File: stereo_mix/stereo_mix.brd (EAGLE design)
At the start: 49 x 100 mm, 16 parts, among them U1 THONKICONNNEW, U2 THONKICONNNEW, U3 THONKICONNNEW, U4 THONKICONNNEW, U5 THONKICONNNEW, U6 THONKICONNNEW, U7 THONKICONNNEW, U8 THONKICONNNEW

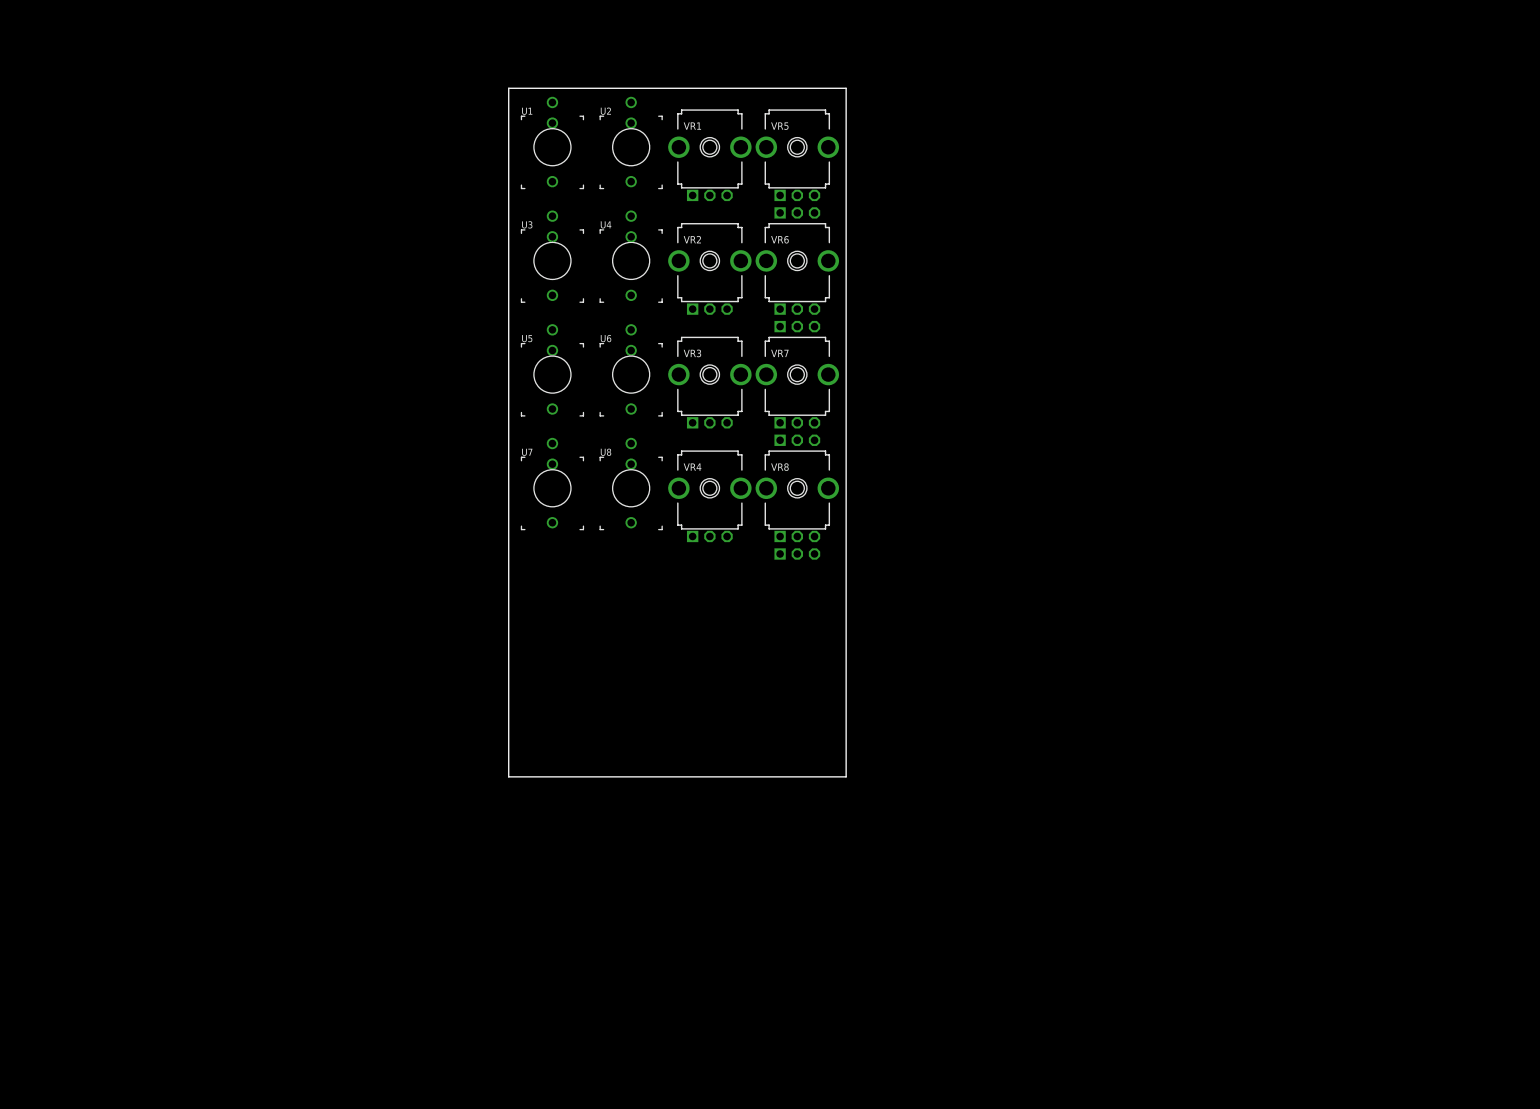
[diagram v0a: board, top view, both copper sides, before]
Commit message: Start implementation of stereo_mixer
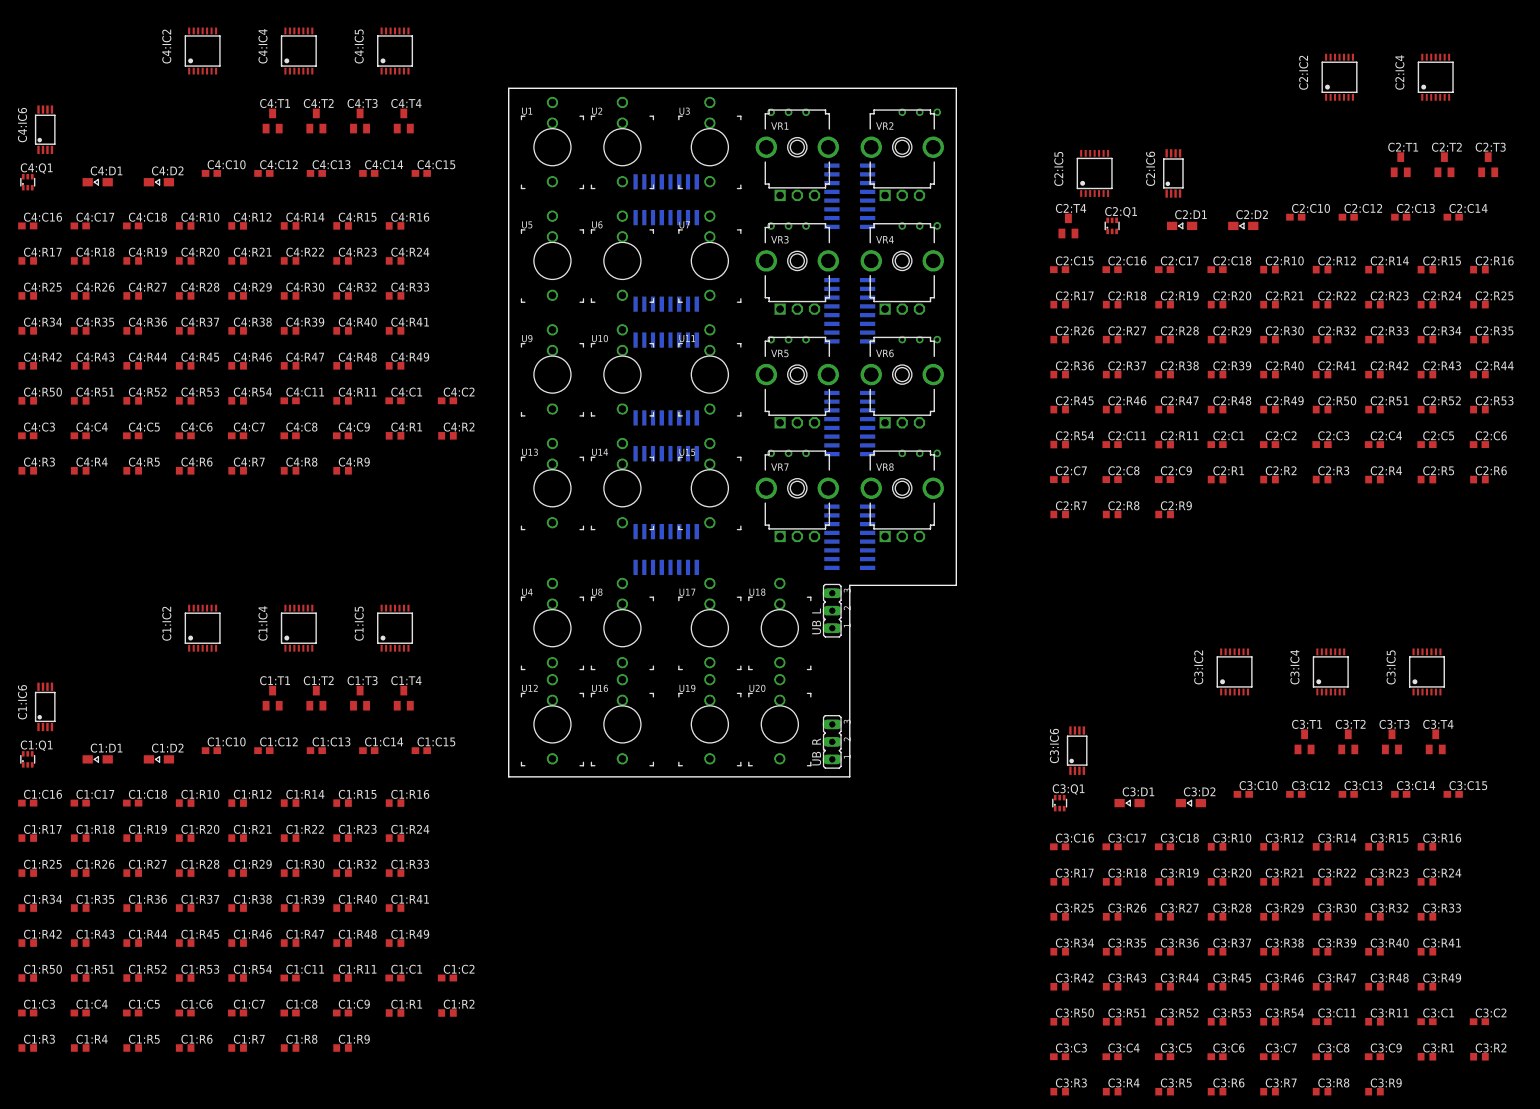
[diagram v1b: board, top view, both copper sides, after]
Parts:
- added C1:C1, C1:C3, C1:C5, C1:C6, C2:C1, C2:C3, C2:C5, C2:C6, C3:C1, C3:C3, C3:C5, C3:C6, C4:C1, C4:C3, C4:C5, C4:C6: 100pF, rcl:C0603
- added C1:C10, C1:C11, C1:C12, C1:C13, C1:C14, C1:C15, C1:C16, C1:C17, C1:C18, C1:C7, C1:C8, C1:C9, C2:C10, C2:C11, C2:C12, C2:C13, C2:C14, C2:C15, C2:C16, C2:C17, C2:C18, C2:C7, C2:C8, C2:C9, C3:C10, C3:C11, C3:C12, C3:C13, C3:C14, C3:C15, C3:C16, C3:C17, C3:C18, C3:C7, C3:C8, C3:C9, C4:C10, C4:C11, C4:C12, C4:C13, C4:C14, C4:C15, C4:C16, C4:C17, C4:C18, C4:C7, C4:C8, C4:C9: 100nF, rcl:C0603
- added C1:C2, C1:C4, C2:C2, C2:C4, C3:C2, C3:C4, C4:C2, C4:C4: 22pF, rcl:C0603
- added C1:D1, C1:D2, C2:D1, C2:D2, C3:D1, C3:D2, C4:D1, C4:D2: 1N4148, diode:SOD323-W
- added C1:IC1, C1:IC3, C2:IC1, C2:IC3, C3:IC1, C3:IC3, C4:IC1, C4:IC3: LM13700M, ota:SO16
- added C1:IC2, C1:IC4, C1:IC5, C2:IC2, C2:IC4, C2:IC5, C3:IC2, C3:IC4, C3:IC5, C4:IC2, C4:IC4, C4:IC5: TL084PW, op-amp:TSSOP14
- added C1:IC6, C2:IC6, C3:IC6, C4:IC6: TL082PW, op-amp:TSSOP8
- added C1:Q1, C2:Q1, C3:Q1, C4:Q1: BC847BS, transistor-small-signal:SOT363_PHILIPS
- added C1:R1, C1:R19, C2:R1, C2:R19, C3:R1, C3:R19, C4:R1, C4:R19: 22, rcl:R0603
- added C1:R10, C1:R15, C1:R28, C1:R33, C1:R43, C1:R44, C1:R45, C1:R46, C1:R49, C1:R50, C1:R51, C1:R52, C1:R53, C1:R54, C2:R10, C2:R15, C2:R28, C2:R33, C2:R43, C2:R44, C2:R45, C2:R46, C2:R49, C2:R50, C2:R51, C2:R52, C2:R53, C2:R54, C3:R10, C3:R15, C3:R28, C3:R33, C3:R43, C3:R44, C3:R45, C3:R46, C3:R49, C3:R50, C3:R51, C3:R52, C3:R53, C3:R54, C4:R10, C4:R15, C4:R28, C4:R33, C4:R43, C4:R44, C4:R45, C4:R46, C4:R49, C4:R50, C4:R51, C4:R52, C4:R53, C4:R54: 100k, rcl:R0603
- added C1:R11, C1:R29, C2:R11, C2:R29, C3:R11, C3:R29, C4:R11, C4:R29: 680, rcl:R0603
- added C1:R12, C1:R30, C1:R37, C1:R39, C2:R12, C2:R30, C2:R37, C2:R39, C3:R12, C3:R30, C3:R37, C3:R39, C4:R12, C4:R30, C4:R37, C4:R39: 1M, rcl:R0603
- added C1:R13, C1:R31, C2:R13, C2:R31, C3:R13, C3:R31, C4:R13, C4:R31: 100k, rcl:RTRIMT93YA
- added C1:R14, C1:R32, C2:R14, C2:R32, C3:R14, C3:R32, C4:R14, C4:R32: 47k, rcl:R0603
- added C1:R16, C1:R34, C2:R16, C2:R34, C3:R16, C3:R34, C4:R16, C4:R34: 68k, rcl:R0603
- added C1:R17, C1:R27, C1:R35, C1:R9, C2:R17, C2:R27, C2:R35, C2:R9, C3:R17, C3:R27, C3:R35, C3:R9, C4:R17, C4:R27, C4:R35, C4:R9: 15k, rcl:R0603
- added C1:R18, C1:R36, C2:R18, C2:R36, C3:R18, C3:R36, C4:R18, C4:R36: 680k, rcl:R0603
- added C1:R2, C1:R20, C2:R2, C2:R20, C3:R2, C3:R20, C4:R2, C4:R20: 470, rcl:R0603
- added C1:R21, C1:R3, C2:R21, C2:R3, C3:R21, C3:R3, C4:R21, C4:R3: 510, rcl:R0603
- added C1:R22, C1:R4, C2:R22, C2:R4, C3:R22, C3:R4, C4:R22, C4:R4: 21k, rcl:R0603
- added C1:R23, C1:R5, C2:R23, C2:R5, C3:R23, C3:R5, C4:R23, C4:R5: 12k, rcl:R0603
- added C1:R24, C1:R6, C2:R24, C2:R6, C3:R24, C3:R6, C4:R24, C4:R6: 7k2, rcl:R0603
- added C1:R25, C1:R7, C2:R25, C2:R7, C3:R25, C3:R7, C4:R25, C4:R7: 6k8, rcl:R0603
- added C1:R26, C1:R8, C2:R26, C2:R8, C3:R26, C3:R8, C4:R26, C4:R8: 560, rcl:R0603
- added C1:R38, C2:R38, C3:R38, C4:R38: 1k, rcl:R0603
- added C1:R40, C2:R40, C3:R40, C4:R40: 10k, rcl:R0603
- added C1:R41, C2:R41, C3:R41, C4:R41: 10M, rcl:R0603
- added C1:R42, C2:R42, C3:R42, C4:R42: 1k5, rcl:R0603
- added C1:R47, C1:R48, C2:R47, C2:R48, C3:R47, C3:R48, C4:R47, C4:R48: 200k, rcl:R0603
- added C1:T1, C1:T2, C1:T3, C1:T4, C2:T1, C2:T2, C2:T3, C2:T4, C3:T1, C3:T2, C3:T3, C3:T4, C4:T1, C4:T2, C4:T3, C4:T4: 3906, transistor-neu-to92:SOT23-BEC
- added U10, U11, U12, U13, U14, U15, U16, U17, U18, U19, U20, U9: THONKICONNNEW, MusicThingModular:WQP-PJ301M-12_JACK
- added UB_L, UB_R: (no value), jumper:JP2
- VR5, VR6, VR7, VR8: device MusicThingModular:DUAL_9MM_SNAP-IN_POT -> MusicThingModular:9MM_SNAP-IN_POT
- moved U4 54.6 mm to (6.35, 21.6)
- moved VR4 43.3 mm to (57.1, 74.9)
- moved U7 40.2 mm to (29.2, 74.9)
- moved VR5 33.0 mm to (41.9, 58.4)
- moved VR2 32.5 mm to (57.1, 91.4)
- moved U3 28.2 mm to (29.2, 91.4)
- moved VR6 22.5 mm to (57.1, 58.4)
- moved VR3 20.8 mm to (41.9, 74.9)
- moved U8 20.4 mm to (16.5, 21.6)
- moved U6 16.6 mm to (16.5, 74.9)
- moved U5 16.5 mm to (6.35, 74.9)
- moved VR7 16.5 mm to (41.9, 41.9)
- moved VR8 15.2 mm to (57.1, 41.9)
- moved VR1 12.7 mm to (41.9, 91.4)
- moved U2 1.27 mm to (16.5, 91.4)
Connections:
- new net +12V: C1:C10.2, C1:C11.2, C1:C12.2, C1:C7.2, C1:C8.2, C1:C9.2, C1:IC1.11, C1:IC2.4, C1:IC3.11, C1:IC4.4, C1:IC5.4, C1:IC6.8, C1:R13.1, C1:R23.1, C1:R31.1, C1:R37.2, C1:R41.2, C1:R5.1, C2:C10.2, C2:C11.2, C2:C12.2, C2:C7.2, C2:C8.2, C2:C9.2, C2:IC1.11, C2:IC2.4, C2:IC3.11, C2:IC4.4, C2:IC5.4, C2:IC6.8, C2:R13.1, C2:R23.1, C2:R31.1, C2:R37.2, C2:R41.2, C2:R5.1, C3:C10.2, C3:C11.2, C3:C12.2, C3:C7.2, C3:C8.2, C3:C9.2, C3:IC1.11, C3:IC2.4, C3:IC3.11, C3:IC4.4, C3:IC5.4, C3:IC6.8, C3:R13.1, C3:R23.1, C3:R31.1, C3:R37.2, C3:R41.2, C3:R5.1, C4:C10.2, C4:C11.2, C4:C12.2, C4:C7.2, C4:C8.2, C4:C9.2, C4:IC1.11, C4:IC2.4, C4:IC3.11, C4:IC4.4, C4:IC5.4, C4:IC6.8, C4:R13.1, C4:R23.1, C4:R31.1, C4:R37.2, C4:R41.2, C4:R5.1
- new net -12V: C1:C13.1, C1:C14.1, C1:C15.1, C1:C16.1, C1:C17.1, C1:C18.1, C1:IC1.6, C1:IC2.11, C1:IC3.6, C1:IC4.11, C1:IC5.11, C1:IC6.4, C1:R13.3, C1:R18.2, C1:R31.3, C1:R36.2, C2:C13.1, C2:C14.1, C2:C15.1, C2:C16.1, C2:C17.1, C2:C18.1, C2:IC1.6, C2:IC2.11, C2:IC3.6, C2:IC4.11, C2:IC5.11, C2:IC6.4, C2:R13.3, C2:R18.2, C2:R31.3, C2:R36.2, C3:C13.1, C3:C14.1, C3:C15.1, C3:C16.1, C3:C17.1, C3:C18.1, C3:IC1.6, C3:IC2.11, C3:IC3.6, C3:IC4.11, C3:IC5.11, C3:IC6.4, C3:R13.3, C3:R18.2, C3:R31.3, C3:R36.2, C4:C13.1, C4:C14.1, C4:C15.1, C4:C16.1, C4:C17.1, C4:C18.1, C4:IC1.6, C4:IC2.11, C4:IC3.6, C4:IC4.11, C4:IC5.11, C4:IC6.4, C4:R13.3, C4:R18.2, C4:R31.3, C4:R36.2
- new net C1:N$1: C1:IC1.4, C1:R1.2
- new net C1:N$10: C1:R8.1, C1:R9.2
- new net C1:N$11: C1:IC2.7, C1:R10.1, C1:R8.2
- new net C1:N$12: C1:C1.1, C1:IC1.13, C1:R12.2, C1:R14.1
- new net C1:N$13: C1:IC1.14, C1:R10.2, C1:R11.2
- new net C1:N$14: C1:R12.1, C1:R13.2
- new net C1:N$15: C1:C2.1, C1:IC2.9, C1:R15.1, C1:R16.2
- new net C1:N$16: C1:C1.2, C1:IC1.12, C1:IC2.10, C1:R14.2
- new net C1:N$17: C1:IC1.16, C1:R17.2
- new net C1:N$18: C1:R17.1, C1:R18.1, C1:T2.C
- new net C1:N$19: C1:IC2.13, C1:IC2.14, C1:T2.B
- new net C1:N$2: C1:R1.1, C1:R2.2
- new net C1:N$20: C1:IC3.4, C1:R19.2
- new net C1:N$21: C1:R19.1, C1:R20.2
- new net C1:N$22: C1:IC3.3, C1:R21.2, C1:R22.2
- new net C1:N$23: C1:IC3.2, C1:R23.2
- new net C1:N$24: C1:IC3.1, C1:R24.2
- new net C1:N$25: C1:R24.1, C1:T3.C
- new net C1:N$26: C1:D2.A, C1:IC4.1, C1:T3.B
- new net C1:N$27: C1:D2.C, C1:IC4.2, C1:R25.2, C1:T3.E
- new net C1:N$28: C1:IC3.5, C1:IC4.6, C1:R27.1
- new net C1:N$29: C1:R26.1, C1:R27.2
- new net C1:N$3: C1:IC1.3, C1:R3.2, C1:R4.2
- new net C1:N$30: C1:IC4.7, C1:R26.2, C1:R28.1
- new net C1:N$31: C1:IC3.14, C1:R28.2, C1:R29.2
- new net C1:N$32: C1:C3.1, C1:IC3.13, C1:R30.2, C1:R32.1
- new net C1:N$33: C1:R30.1, C1:R31.2
- new net C1:N$34: C1:C3.2, C1:IC3.12, C1:IC4.10, C1:R32.2
- new net C1:N$35: C1:C4.1, C1:IC4.9, C1:R33.1, C1:R34.2
- new net C1:N$36: C1:IC3.16, C1:R35.2
- new net C1:N$37: C1:R35.1, C1:R36.1, C1:T4.C
- new net C1:N$38: C1:IC4.13, C1:IC4.14, C1:T4.B
- new net C1:N$39: C1:IC5.1, C1:IC5.2, C1:R39.2
- new net C1:N$4: C1:IC1.1, C1:R6.2
- new net C1:N$40: C1:IC5.3, C1:R37.1, C1:R38.1
- new net C1:N$41: C1:C5.1, C1:IC5.6, C1:R39.1, C1:R40.1
- new net C1:N$42: C1:C5.2, C1:IC5.7, C1:Q1.2, C1:R40.2
- new net C1:N$43: C1:IC6.5, C1:R43.2, C1:R44.2
- new net C1:N$44: C1:C6.1, C1:IC5.9, C1:Q1.6, C1:R41.1
- new net C1:N$45: C1:IC6.6, C1:R45.2, C1:R46.1
- new net C1:N$46: C1:Q1.1, C1:Q1.4, C1:R42.2
- new net C1:N$47: C1:IC6.2, C1:R47.1, C1:R48.2
- new net C1:N$48: C1:IC5.13, C1:R51.2, C1:R52.1
- new net C1:N$5: C1:IC1.2, C1:R5.2
- new net C1:N$50: C1:IC6.3, C1:R49.2, C1:R50.2
- new net C1:N$6: C1:R6.1, C1:T1.C
- new net C1:N$7: C1:D1.A, C1:IC2.1, C1:T1.B
- new net C1:N$8: C1:D1.C, C1:IC2.2, C1:R7.2, C1:T1.E
- new net C1:N$9: C1:IC1.5, C1:IC2.6, C1:R9.1
- new net C1:OUT_L: C1:C2.2, C1:IC2.8, C1:R15.2
- new net C1:OUT_R: C1:C4.2, C1:IC4.8, C1:R33.2
- new net C1:PAN_CV: C1:IC5.14, C1:R45.1, C1:R49.1, C1:R51.1
- new net C1:PAN_CV_L: C1:IC6.7, C1:R46.2, C1:R7.1
- new net C1:PAN_CV_R: C1:IC6.1, C1:R25.1, C1:R47.2
- new net C1:REF_5: C1:R43.1, C1:R50.1
- new net C1:VOLUME_CV_LOG: C1:C6.2, C1:IC2.12, C1:IC4.12, C1:IC5.8, C1:R42.1
- new net C2:N$1: C2:IC1.4, C2:R1.2
- new net C2:N$10: C2:R8.1, C2:R9.2
- new net C2:N$11: C2:IC2.7, C2:R10.1, C2:R8.2
- new net C2:N$12: C2:C1.1, C2:IC1.13, C2:R12.2, C2:R14.1
- new net C2:N$13: C2:IC1.14, C2:R10.2, C2:R11.2
- new net C2:N$14: C2:R12.1, C2:R13.2
- new net C2:N$15: C2:C2.1, C2:IC2.9, C2:R15.1, C2:R16.2
- new net C2:N$16: C2:C1.2, C2:IC1.12, C2:IC2.10, C2:R14.2
- new net C2:N$17: C2:IC1.16, C2:R17.2
- new net C2:N$18: C2:R17.1, C2:R18.1, C2:T2.C
- new net C2:N$19: C2:IC2.13, C2:IC2.14, C2:T2.B
- new net C2:N$2: C2:R1.1, C2:R2.2
- new net C2:N$20: C2:IC3.4, C2:R19.2
- new net C2:N$21: C2:R19.1, C2:R20.2
- new net C2:N$22: C2:IC3.3, C2:R21.2, C2:R22.2
- new net C2:N$23: C2:IC3.2, C2:R23.2
- new net C2:N$24: C2:IC3.1, C2:R24.2
- new net C2:N$25: C2:R24.1, C2:T3.C
- new net C2:N$26: C2:D2.A, C2:IC4.1, C2:T3.B
- new net C2:N$27: C2:D2.C, C2:IC4.2, C2:R25.2, C2:T3.E
- new net C2:N$28: C2:IC3.5, C2:IC4.6, C2:R27.1
- new net C2:N$29: C2:R26.1, C2:R27.2
- new net C2:N$3: C2:IC1.3, C2:R3.2, C2:R4.2
- new net C2:N$30: C2:IC4.7, C2:R26.2, C2:R28.1
- new net C2:N$31: C2:IC3.14, C2:R28.2, C2:R29.2
- new net C2:N$32: C2:C3.1, C2:IC3.13, C2:R30.2, C2:R32.1
- new net C2:N$33: C2:R30.1, C2:R31.2
- new net C2:N$34: C2:C3.2, C2:IC3.12, C2:IC4.10, C2:R32.2
- new net C2:N$35: C2:C4.1, C2:IC4.9, C2:R33.1, C2:R34.2
- new net C2:N$36: C2:IC3.16, C2:R35.2
- new net C2:N$37: C2:R35.1, C2:R36.1, C2:T4.C
- new net C2:N$38: C2:IC4.13, C2:IC4.14, C2:T4.B
- new net C2:N$39: C2:IC5.1, C2:IC5.2, C2:R39.2
- new net C2:N$4: C2:IC1.1, C2:R6.2
- new net C2:N$40: C2:IC5.3, C2:R37.1, C2:R38.1
- new net C2:N$41: C2:C5.1, C2:IC5.6, C2:R39.1, C2:R40.1
- new net C2:N$42: C2:C5.2, C2:IC5.7, C2:Q1.2, C2:R40.2
- new net C2:N$43: C2:IC6.5, C2:R43.2, C2:R44.2
- new net C2:N$44: C2:C6.1, C2:IC5.9, C2:Q1.6, C2:R41.1
- new net C2:N$45: C2:IC6.6, C2:R45.2, C2:R46.1
- new net C2:N$46: C2:Q1.1, C2:Q1.4, C2:R42.2
- new net C2:N$47: C2:IC6.2, C2:R47.1, C2:R48.2
- new net C2:N$48: C2:IC5.13, C2:R51.2, C2:R52.1
- new net C2:N$5: C2:IC1.2, C2:R5.2
- new net C2:N$50: C2:IC6.3, C2:R49.2, C2:R50.2
- new net C2:N$6: C2:R6.1, C2:T1.C
- new net C2:N$7: C2:D1.A, C2:IC2.1, C2:T1.B
- new net C2:N$8: C2:D1.C, C2:IC2.2, C2:R7.2, C2:T1.E
- new net C2:N$9: C2:IC1.5, C2:IC2.6, C2:R9.1
- new net C2:OUT_L: C2:C2.2, C2:IC2.8, C2:R15.2
- new net C2:OUT_R: C2:C4.2, C2:IC4.8, C2:R33.2
- new net C2:PAN_CV: C2:IC5.14, C2:R45.1, C2:R49.1, C2:R51.1
- new net C2:PAN_CV_L: C2:IC6.7, C2:R46.2, C2:R7.1
- new net C2:PAN_CV_R: C2:IC6.1, C2:R25.1, C2:R47.2
- new net C2:REF_5: C2:R43.1, C2:R50.1
- new net C2:VOLUME_CV_LOG: C2:C6.2, C2:IC2.12, C2:IC4.12, C2:IC5.8, C2:R42.1
- new net C3:N$1: C3:IC1.4, C3:R1.2
- new net C3:N$10: C3:R8.1, C3:R9.2
- new net C3:N$11: C3:IC2.7, C3:R10.1, C3:R8.2
- new net C3:N$12: C3:C1.1, C3:IC1.13, C3:R12.2, C3:R14.1
- new net C3:N$13: C3:IC1.14, C3:R10.2, C3:R11.2
- new net C3:N$14: C3:R12.1, C3:R13.2
- new net C3:N$15: C3:C2.1, C3:IC2.9, C3:R15.1, C3:R16.2
- new net C3:N$16: C3:C1.2, C3:IC1.12, C3:IC2.10, C3:R14.2
- new net C3:N$17: C3:IC1.16, C3:R17.2
- new net C3:N$18: C3:R17.1, C3:R18.1, C3:T2.C
- new net C3:N$19: C3:IC2.13, C3:IC2.14, C3:T2.B
- new net C3:N$2: C3:R1.1, C3:R2.2
- new net C3:N$20: C3:IC3.4, C3:R19.2
- new net C3:N$21: C3:R19.1, C3:R20.2
- new net C3:N$22: C3:IC3.3, C3:R21.2, C3:R22.2
- new net C3:N$23: C3:IC3.2, C3:R23.2
- new net C3:N$24: C3:IC3.1, C3:R24.2
- new net C3:N$25: C3:R24.1, C3:T3.C
- new net C3:N$26: C3:D2.A, C3:IC4.1, C3:T3.B
- new net C3:N$27: C3:D2.C, C3:IC4.2, C3:R25.2, C3:T3.E
- new net C3:N$28: C3:IC3.5, C3:IC4.6, C3:R27.1
- new net C3:N$29: C3:R26.1, C3:R27.2
- new net C3:N$3: C3:IC1.3, C3:R3.2, C3:R4.2
- new net C3:N$30: C3:IC4.7, C3:R26.2, C3:R28.1
- new net C3:N$31: C3:IC3.14, C3:R28.2, C3:R29.2
- new net C3:N$32: C3:C3.1, C3:IC3.13, C3:R30.2, C3:R32.1
- new net C3:N$33: C3:R30.1, C3:R31.2
- new net C3:N$34: C3:C3.2, C3:IC3.12, C3:IC4.10, C3:R32.2
- new net C3:N$35: C3:C4.1, C3:IC4.9, C3:R33.1, C3:R34.2
- new net C3:N$36: C3:IC3.16, C3:R35.2
- new net C3:N$37: C3:R35.1, C3:R36.1, C3:T4.C
- new net C3:N$38: C3:IC4.13, C3:IC4.14, C3:T4.B
- new net C3:N$39: C3:IC5.1, C3:IC5.2, C3:R39.2
- new net C3:N$4: C3:IC1.1, C3:R6.2
- new net C3:N$40: C3:IC5.3, C3:R37.1, C3:R38.1
- new net C3:N$41: C3:C5.1, C3:IC5.6, C3:R39.1, C3:R40.1
- new net C3:N$42: C3:C5.2, C3:IC5.7, C3:Q1.2, C3:R40.2
- new net C3:N$43: C3:IC6.5, C3:R43.2, C3:R44.2
- new net C3:N$44: C3:C6.1, C3:IC5.9, C3:Q1.6, C3:R41.1
- new net C3:N$45: C3:IC6.6, C3:R45.2, C3:R46.1
- new net C3:N$46: C3:Q1.1, C3:Q1.4, C3:R42.2
- new net C3:N$47: C3:IC6.2, C3:R47.1, C3:R48.2
- new net C3:N$48: C3:IC5.13, C3:R51.2, C3:R52.1
- new net C3:N$5: C3:IC1.2, C3:R5.2
- new net C3:N$50: C3:IC6.3, C3:R49.2, C3:R50.2
- new net C3:N$6: C3:R6.1, C3:T1.C
- new net C3:N$7: C3:D1.A, C3:IC2.1, C3:T1.B
- new net C3:N$8: C3:D1.C, C3:IC2.2, C3:R7.2, C3:T1.E
- new net C3:N$9: C3:IC1.5, C3:IC2.6, C3:R9.1
- new net C3:OUT_L: C3:C2.2, C3:IC2.8, C3:R15.2
- new net C3:OUT_R: C3:C4.2, C3:IC4.8, C3:R33.2
- new net C3:PAN_CV: C3:IC5.14, C3:R45.1, C3:R49.1, C3:R51.1
- new net C3:PAN_CV_L: C3:IC6.7, C3:R46.2, C3:R7.1
- new net C3:PAN_CV_R: C3:IC6.1, C3:R25.1, C3:R47.2
- new net C3:REF_5: C3:R43.1, C3:R50.1
- new net C3:VOLUME_CV_LOG: C3:C6.2, C3:IC2.12, C3:IC4.12, C3:IC5.8, C3:R42.1
- new net C4:N$1: C4:IC1.4, C4:R1.2
- new net C4:N$10: C4:R8.1, C4:R9.2
- new net C4:N$11: C4:IC2.7, C4:R10.1, C4:R8.2
- new net C4:N$12: C4:C1.1, C4:IC1.13, C4:R12.2, C4:R14.1
- new net C4:N$13: C4:IC1.14, C4:R10.2, C4:R11.2
- new net C4:N$14: C4:R12.1, C4:R13.2
- new net C4:N$15: C4:C2.1, C4:IC2.9, C4:R15.1, C4:R16.2
- new net C4:N$16: C4:C1.2, C4:IC1.12, C4:IC2.10, C4:R14.2
- new net C4:N$17: C4:IC1.16, C4:R17.2
- new net C4:N$18: C4:R17.1, C4:R18.1, C4:T2.C
- new net C4:N$19: C4:IC2.13, C4:IC2.14, C4:T2.B
- new net C4:N$2: C4:R1.1, C4:R2.2
- new net C4:N$20: C4:IC3.4, C4:R19.2
- new net C4:N$21: C4:R19.1, C4:R20.2
- new net C4:N$22: C4:IC3.3, C4:R21.2, C4:R22.2
- new net C4:N$23: C4:IC3.2, C4:R23.2
- new net C4:N$24: C4:IC3.1, C4:R24.2
- new net C4:N$25: C4:R24.1, C4:T3.C
- new net C4:N$26: C4:D2.A, C4:IC4.1, C4:T3.B
- new net C4:N$27: C4:D2.C, C4:IC4.2, C4:R25.2, C4:T3.E
- new net C4:N$28: C4:IC3.5, C4:IC4.6, C4:R27.1
- new net C4:N$29: C4:R26.1, C4:R27.2
- new net C4:N$3: C4:IC1.3, C4:R3.2, C4:R4.2
- new net C4:N$30: C4:IC4.7, C4:R26.2, C4:R28.1
- new net C4:N$31: C4:IC3.14, C4:R28.2, C4:R29.2
- new net C4:N$32: C4:C3.1, C4:IC3.13, C4:R30.2, C4:R32.1
- new net C4:N$33: C4:R30.1, C4:R31.2
- new net C4:N$34: C4:C3.2, C4:IC3.12, C4:IC4.10, C4:R32.2
- new net C4:N$35: C4:C4.1, C4:IC4.9, C4:R33.1, C4:R34.2
- new net C4:N$36: C4:IC3.16, C4:R35.2
- new net C4:N$37: C4:R35.1, C4:R36.1, C4:T4.C
- new net C4:N$38: C4:IC4.13, C4:IC4.14, C4:T4.B
- new net C4:N$39: C4:IC5.1, C4:IC5.2, C4:R39.2
- new net C4:N$4: C4:IC1.1, C4:R6.2
- new net C4:N$40: C4:IC5.3, C4:R37.1, C4:R38.1
- new net C4:N$41: C4:C5.1, C4:IC5.6, C4:R39.1, C4:R40.1
- new net C4:N$42: C4:C5.2, C4:IC5.7, C4:Q1.2, C4:R40.2
- new net C4:N$43: C4:IC6.5, C4:R43.2, C4:R44.2
- new net C4:N$44: C4:C6.1, C4:IC5.9, C4:Q1.6, C4:R41.1
- new net C4:N$45: C4:IC6.6, C4:R45.2, C4:R46.1
- new net C4:N$46: C4:Q1.1, C4:Q1.4, C4:R42.2
- new net C4:N$47: C4:IC6.2, C4:R47.1, C4:R48.2
- new net C4:N$48: C4:IC5.13, C4:R51.2, C4:R52.1
- new net C4:N$5: C4:IC1.2, C4:R5.2
- new net C4:N$50: C4:IC6.3, C4:R49.2, C4:R50.2
- new net C4:N$6: C4:R6.1, C4:T1.C
- new net C4:N$7: C4:D1.A, C4:IC2.1, C4:T1.B
- new net C4:N$8: C4:D1.C, C4:IC2.2, C4:R7.2, C4:T1.E
- new net C4:N$9: C4:IC1.5, C4:IC2.6, C4:R9.1
- new net C4:OUT_L: C4:C2.2, C4:IC2.8, C4:R15.2
- new net C4:OUT_R: C4:C4.2, C4:IC4.8, C4:R33.2
- new net C4:PAN_CV: C4:IC5.14, C4:R45.1, C4:R49.1, C4:R51.1
- new net C4:PAN_CV_L: C4:IC6.7, C4:R46.2, C4:R7.1
- new net C4:PAN_CV_R: C4:IC6.1, C4:R25.1, C4:R47.2
- new net C4:REF_5: C4:R43.1, C4:R50.1
- new net C4:VOLUME_CV_LOG: C4:C6.2, C4:IC2.12, C4:IC4.12, C4:IC5.8, C4:R42.1
- new net N$17: U4.P$1_TIP, VR2.3
- new net N$18: C3:R52.2, C3:R53.1, U11.P$1_TIP, VR5.3
- new net N$19: C3:R54.2, VR5.1
- new net N$20: C3:R38.2, VR6.2
- new net N$21: U12.P$1_TIP, VR6.3
- new net N$22: C4:R4.1, U13.P$1_TIP, U14.P$2_SWITCH
- new net N$23: C4:R22.1, U14.P$1_TIP
- new net N$24: C4:IC5.12, C4:R53.2, C4:R54.1, VR7.2
- new net N$25: C4:R52.2, C4:R53.1, U15.P$1_TIP, VR7.3
- new net N$26: C4:R54.2, VR7.1
- new net N$27: C4:R38.2, VR8.2
- new net N$28: U16.P$1_TIP, VR8.3
- new net N$29: U17.P$1_TIP
- new net N$30: U18.P$1_TIP
- new net N$31: U18.P$2_SWITCH, U20.P$1_TIP
- new net N$32: U17.P$2_SWITCH, U19.P$1_TIP
- new net REF_10: U12.P$2_SWITCH, U16.P$2_SWITCH, U4.P$2_SWITCH, U8.P$2_SWITCH
- new net REF_5: U11.P$2_SWITCH, U15.P$2_SWITCH, U3.P$2_SWITCH, U7.P$2_SWITCH
- net GND: now also C1:C10.1, C1:C11.1, C1:C12.1, C1:C13.2, C1:C14.2, C1:C15.2, C1:C16.2, C1:C17.2, C1:C18.2, C1:C7.1, C1:C8.1, C1:C9.1, C1:IC2.3, C1:IC2.5, C1:IC4.3, C1:IC4.5, C1:IC5.10, C1:IC5.5, C1:Q1.3, C1:Q1.5, C1:R11.1, C1:R16.1, C1:R2.1, C1:R20.1, C1:R21.1, C1:R29.1, C1:R3.1, C1:R34.1, C1:R44.1, C1:R48.1, C1:T2.E, C1:T4.E, C2:C10.1, C2:C11.1, C2:C12.1, C2:C13.2, C2:C14.2, C2:C15.2, C2:C16.2, C2:C17.2, C2:C18.2, C2:C7.1, C2:C8.1, C2:C9.1, C2:IC2.3, C2:IC2.5, C2:IC4.3, C2:IC4.5, C2:IC5.10, C2:IC5.5, C2:Q1.3, C2:Q1.5, C2:R11.1, C2:R16.1, C2:R2.1, C2:R20.1, C2:R21.1, C2:R29.1, C2:R3.1, C2:R34.1, C2:R44.1, C2:R48.1, C2:T2.E, C2:T4.E, C3:C10.1, C3:C11.1, C3:C12.1, C3:C13.2, C3:C14.2, C3:C15.2, C3:C16.2, C3:C17.2, C3:C18.2, C3:C7.1, C3:C8.1, C3:C9.1, C3:IC2.3, C3:IC2.5, C3:IC4.3, C3:IC4.5, C3:IC5.10, C3:IC5.5, C3:Q1.3, C3:Q1.5, C3:R11.1, C3:R16.1, C3:R2.1, C3:R20.1, C3:R21.1, C3:R29.1, C3:R3.1, C3:R34.1, C3:R44.1, C3:R48.1, C3:T2.E, C3:T4.E, C4:C10.1, C4:C11.1, C4:C12.1, C4:C13.2, C4:C14.2, C4:C15.2, C4:C16.2, C4:C17.2, C4:C18.2, C4:C7.1, C4:C8.1, C4:C9.1, C4:IC2.3, C4:IC2.5, C4:IC4.3, C4:IC4.5, C4:IC5.10, C4:IC5.5, C4:Q1.3, C4:Q1.5, C4:R11.1, C4:R16.1, C4:R2.1, C4:R20.1, C4:R21.1, C4:R29.1, C4:R3.1, C4:R34.1, C4:R44.1, C4:R48.1, C4:T2.E, C4:T4.E, U1.P$3_SLEEVE, U10.P$3_SLEEVE, U11.P$3_SLEEVE, U12.P$3_SLEEVE, U13.P$3_SLEEVE, U14.P$3_SLEEVE, U15.P$3_SLEEVE, U16.P$3_SLEEVE, U17.P$3_SLEEVE, U18.P$3_SLEEVE, U19.P$3_SLEEVE, U2.P$3_SLEEVE, U20.P$3_SLEEVE, U3.P$3_SLEEVE, U4.P$3_SLEEVE, U5.P$3_SLEEVE, U6.P$3_SLEEVE, U7.P$3_SLEEVE, U8.P$3_SLEEVE, U9.P$3_SLEEVE, VR2.1, VR4.1; no longer VR1.2, VR2.2, VR3.2, VR4.2, VR5.1, VR5.1B, VR6.1B, VR7.1, VR7.1B, VR8.1B
- net N$1: now also C1:R4.1; no longer VR1.1, VR5.3
- net N$10: now also C2:R52.2, C2:R53.1, U7.P$1_TIP, VR3.3; no longer VR5.2
- net N$11: now also C2:R54.2, VR3.1; no longer VR5.2B
- net N$12: now also C2:R38.2, VR4.2; no longer VR6.2
- net N$13: now also U8.P$1_TIP, VR4.3; no longer VR7.2
- net N$14: now also C3:R4.1, U10.P$2_SWITCH, U9.P$1_TIP; no longer VR7.2B
- net N$15: now also C3:R22.1, U10.P$1_TIP; no longer VR8.2
- net N$16: now also C3:IC5.12, C3:R53.2, C3:R54.1, VR5.2; no longer VR8.2B
- net N$2: now also C1:R22.1, U2.P$1_TIP; no longer U3.P$1_TIP, U4.P$2_SWITCH, VR2.1, VR6.3
- net N$3: now also C1:IC5.12, C1:R53.2, C1:R54.1, VR1.2; no longer U5.P$1_TIP, U6.P$2_SWITCH, VR3.1, VR7.3
- net N$4: now also C2:R4.1, U5.P$1_TIP, U6.P$2_SWITCH; no longer U7.P$1_TIP, U8.P$2_SWITCH, VR4.1, VR8.3
- net N$5: now also C1:R52.2, C1:R53.1, U3.P$1_TIP, VR1.3; no longer VR6.2B
- net N$6: now also C1:R54.2, VR1.1; no longer U2.P$1_TIP, VR1.3, VR5.3B
- net N$7: now also C1:R38.2, VR2.2; no longer U4.P$1_TIP, VR2.3, VR6.3B
- net N$8: now also C2:R22.1; no longer VR3.3, VR7.3B
- net N$9: now also C2:IC5.12, C2:R53.2, C2:R54.1, VR3.2; no longer U8.P$1_TIP, VR4.3, VR8.3B
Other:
- board size 49 x 100 mm -> 65 x 100 mm
